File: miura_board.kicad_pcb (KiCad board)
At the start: 2 copper layers, 60 x 60 mm, 27 parts, among them J1 Conn_01x02_Female, J2 Screw_Terminal_01x02, J3 Screw_Terminal_01x02, SW1 SW_Push, U1 ATmega32U4-A, U2 NRF24L01, U3 DRV8833PW, U4 DRV8833PW, U5 ESP32-S2-SOLO, Y1 16MHz, Y2 16MHz

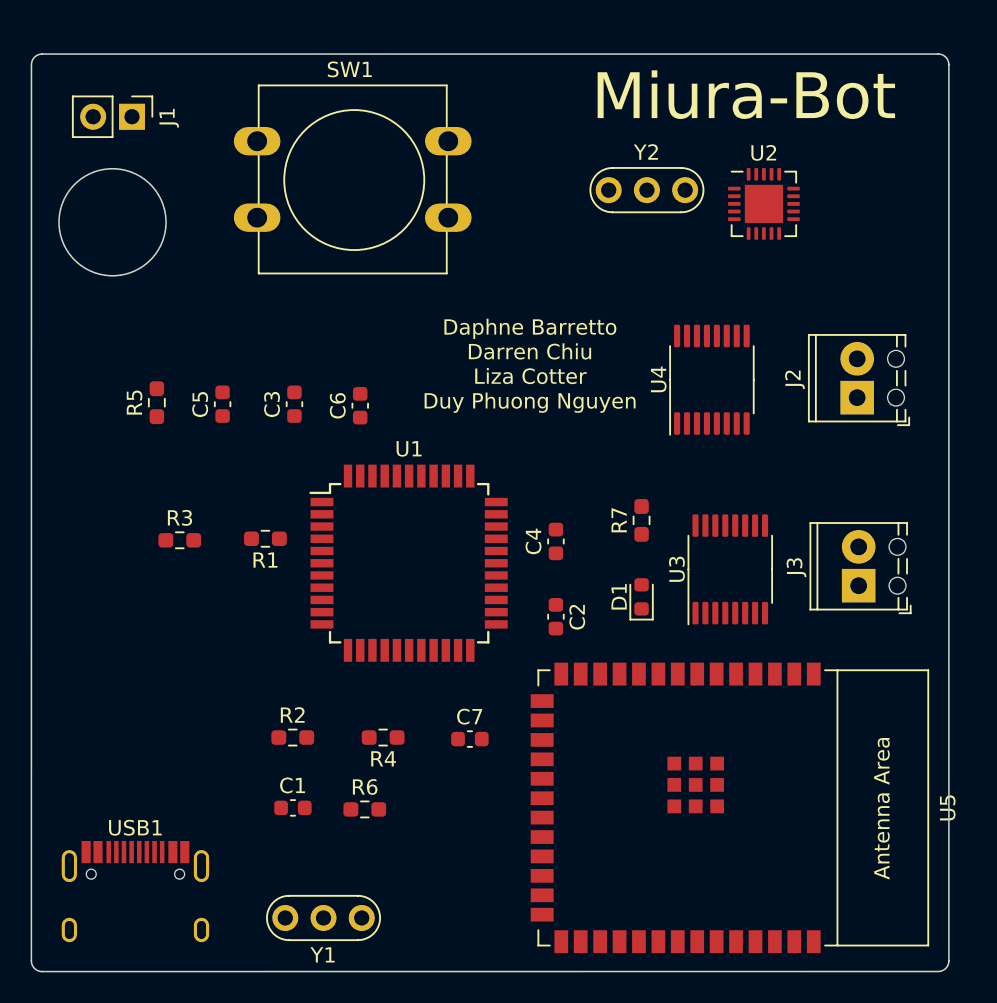
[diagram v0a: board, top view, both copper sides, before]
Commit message: STEP
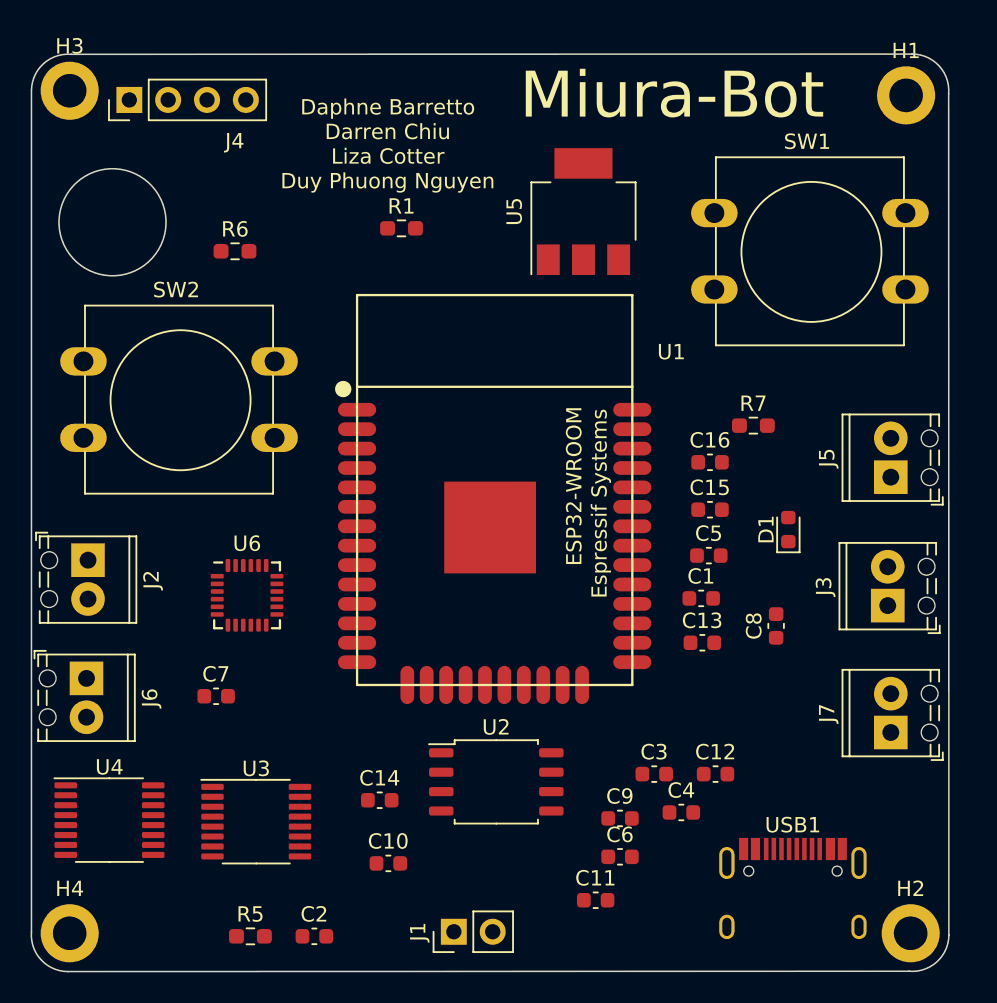
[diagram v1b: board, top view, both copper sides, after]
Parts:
- removed R2: 22, Resistor_SMD:R_0603_1608Metric_Pad0.98x0.95mm_HandSolder
- removed R3, R4: 10k, Resistor_SMD:R_0603_1608Metric_Pad0.98x0.95mm_HandSolder
- removed Y1, Y2: 16MHz, Crystal:Resonator-3Pin_W7.0mm_H2.5mm
- added C10: 0.1uF, Capacitor_SMD:C_0603_1608Metric, F.Cu at (84.3, 77.8)
- added C11: 0.1uF, Capacitor_SMD:C_0603_1608Metric, F.Cu at (97.9, 80.2)
- added C12: 0.1uF, Capacitor_SMD:C_0603_1608Metric, F.Cu at (105.7, 72.0)
- added C13: 0.1uF, Capacitor_SMD:C_0603_1608Metric, F.Cu at (104.9, 63.4)
- added C14: 0.1uF, Capacitor_SMD:C_0603_1608Metric, F.Cu at (83.8, 73.7)
- added C15: 0.1uF, Capacitor_SMD:C_0603_1608Metric, F.Cu at (105.4, 54.7)
- added C16: 0.1uF, Capacitor_SMD:C_0603_1608Metric, F.Cu at (105.4, 51.6)
- added C8: 10uF, Capacitor_SMD:C_0603_1608Metric, F.Cu at (109.7, 62.3)
- added C9: 10uF, Capacitor_SMD:C_0603_1608Metric, F.Cu at (99.5, 74.9)
- added H1: MountingHole_Pad, MountingHole:MountingHole_2.2mm_M2_DIN965_Pad, F.Cu at (118.2, 27.6)
- added H2: MountingHole_Pad, MountingHole:MountingHole_2.2mm_M2_DIN965_Pad, F.Cu at (118.5, 82.4)
- added H3: MountingHole_Pad, MountingHole:MountingHole_2.2mm_M2_DIN965_Pad, F.Cu at (63.5, 27.3)
- added H4: MountingHole_Pad, MountingHole:MountingHole_2.2mm_M2_DIN965_Pad, F.Cu at (63.5, 82.4)
- added J4: Conn_01x04_Male, Connector_PinHeader_2.54mm:PinHeader_1x04_P2.54mm_Vertical, F.Cu at (67.4, 27.9)
- added J5: Screw_Terminal_01x02, TerminalBlock_Phoenix:TerminalBlock_Phoenix_MPT-0,5-2-2.54_1x02_P2.54mm_Horizontal, F.Cu at (117.2, 52.6)
- added J6: Screw_Terminal_01x02, TerminalBlock_Phoenix:TerminalBlock_Phoenix_MPT-0,5-2-2.54_1x02_P2.54mm_Horizontal, F.Cu at (64.6, 65.7)
- added J7: Screw_Terminal_01x02, TerminalBlock_Phoenix:TerminalBlock_Phoenix_MPT-0,5-2-2.54_1x02_P2.54mm_Horizontal, F.Cu at (117.2, 69.3)
- added SW2: SW_Push, Button_Switch_THT:SW_PUSH-12mm, F.Cu at (64.4, 45.0)
- added U6: MPU-6050, Sensor_Motion:InvenSense_QFN-24_4x4mm_P0.5mm, F.Cu at (75.1, 60.3)
- C4: value 0.1uF -> 10uF
- R1: value 22 -> 10k
- U1: value ATmega32U4-A -> ESP32-WROOM; footprint Package_QFP:TQFP-44_10x10mm_P0.8mm -> ESP32-footprints-Lib:ESP32-WROOM
- U2: value NRF24L01 -> W25Q32JVSS; footprint Package_DFN_QFN:QFN-20-1EP_4x4mm_P0.5mm_EP2.5x2.5mm -> Package_SO:SOIC-8_5.23x5.23mm_P1.27mm
- U5: value ESP32-S2-SOLO -> AMS1117; footprint Espressif:ESP32-S2-SOLO -> Package_TO_SOT_SMD:SOT-223-3_TabPin2
- moved J1 57.3 mm to (88.6, 82.3), turned to 90 degrees
- moved J2 51.4 mm to (64.7, 58.0), turned to -90 degrees
- moved U4 48.8 mm to (66.1, 75.0), turned to 0 degrees
- moved USB1 43.0 mm to (110.8, 84.6)
- moved U2 41.7 mm to (91.4, 72.5)
- moved U5 39.6 mm to (97.1, 35.2), turned to 90 degrees
- moved R6 37.5 mm to (74.3, 37.8)
- moved R5 35.4 mm to (75.3, 82.6), turned to 0 degrees
- moved U3 35.1 mm to (75.7, 75.1), turned to 0 degrees
- moved C6 34.0 mm to (99.5, 77.4), turned to 0 degrees
- moved C3 33.7 mm to (101.7, 72.0), turned to 0 degrees
- moved C5 33.3 mm to (105.3, 57.7), turned to 0 degrees
- moved SW1 30.3 mm to (105.7, 35.3)
- moved C1 30.0 mm to (104.8, 60.5)
- moved C2 26.2 mm to (79.5, 82.6), turned to 0 degrees
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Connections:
- C1 pad 1: Net-(C1-Pad1) -> +5V
- C4 pad 1: XTAL1 -> +5V
- C7 pad 1: XTAL2 -> GND
- D1 pad 2: +5V -> +3V3
- J2 pad 1: unconnected-(J2-Pad1) -> Net-(U3-Pad7)
- J2 pad 2: unconnected-(J2-Pad2) -> Net-(U3-Pad5)
- J3 pad 1: unconnected-(J3-Pad1) -> Net-(U4-Pad2)
- J3 pad 2: unconnected-(J3-Pad2) -> Net-(U4-Pad4)
- R1 pad 1: D+ -> +3V3
- R1 pad 2: Net-(R1-Pad2) -> Net-(U1-Pad3)
- SW1 pad 1: GND -> Net-(U1-Pad3)
- SW1 pad 2: RESET -> GND
- U1 pad 1: unconnected-(U1-Pad1) -> GND
- U1 pad 10: unconnected-(U1-Pad10) -> MOTOR_B12_IN
- U1 pad 11: unconnected-(U1-Pad11) -> MOTOR_B11_IN
- U1 pad 12: unconnected-(U1-Pad12) -> MOTOR_A12_IN
- U1 pad 13: RESET -> MOTOR_A11_IN
- U1 pad 14: +5V -> unconnected-(U1-Pad14)
- U1 pad 16: XTAL2 -> unconnected-(U1-Pad16)
- U1 pad 17: XTAL1 -> unconnected-(U1-Pad17)
- U1 pad 19: unconnected-(U1-Pad19) -> SPI_CS
- U1 pad 2: +5V -> +3V3
- U1 pad 20: unconnected-(U1-Pad20) -> SPI_CLK
- U1 pad 21: unconnected-(U1-Pad21) -> MISO
- U1 pad 22: unconnected-(U1-Pad22) -> MOSI
- U1 pad 23: GND -> unconnected-(U1-Pad23)
- U1 pad 24: +5V -> unconnected-(U1-Pad24)
- U1 pad 25: unconnected-(U1-Pad25) -> Net-(U1-Pad25)
- U1 pad 3: Net-(R2-Pad1) -> Net-(U1-Pad3)
- U1 pad 33: Net-(R3-Pad1) -> SDA
- U1 pad 34: +5V -> RXD0
- U1 pad 35: GND -> TXD0
- U1 pad 36: unconnected-(U1-Pad36) -> SCL
- U1 pad 38: unconnected-(U1-Pad38) -> GND
- U1 pad 39: unconnected-(U1-Pad39) -> GND
- U1 pad 4: Net-(R1-Pad2) -> unconnected-(U1-Pad4)
- U1 pad 5: GND -> unconnected-(U1-Pad5)
- U1 pad 6: Net-(C1-Pad1) -> MOTOR_B22_IN
- U1 pad 7: unconnected-(U1-Pad7) -> MOTOR_B21_IN
- U1 pad 8: unconnected-(U1-Pad8) -> MOTOR_A22_IN
- U1 pad 9: unconnected-(U1-Pad9) -> MOTOR_A21_IN
- U2 pad 1: unconnected-(U2-Pad1) -> SPI_CS
- U2 pad 2: unconnected-(U2-Pad2) -> MISO
- U2 pad 4: unconnected-(U2-Pad4) -> GND
- U2 pad 5: unconnected-(U2-Pad5) -> MOSI
- U2 pad 6: unconnected-(U2-Pad6) -> SPI_CLK
- U2 pad 8: unconnected-(U2-Pad8) -> +3V3
- U3 pad 10: unconnected-(U3-Pad10) -> MOTOR_B12_IN
- U3 pad 12: unconnected-(U3-Pad12) -> MOTOR_SUPPLY
- U3 pad 15: unconnected-(U3-Pad15) -> MOTOR_A12_IN
- U3 pad 16: unconnected-(U3-Pad16) -> MOTOR_A11_IN
- U3 pad 2: unconnected-(U3-Pad2) -> Net-(U3-Pad2)
- U3 pad 4: unconnected-(U3-Pad4) -> Net-(U3-Pad4)
- U3 pad 5: unconnected-(U3-Pad5) -> Net-(U3-Pad5)
- U3 pad 7: unconnected-(U3-Pad7) -> Net-(U3-Pad7)
- U3 pad 9: unconnected-(U3-Pad9) -> MOTOR_B11_IN
- U4 pad 10: unconnected-(U4-Pad10) -> MOTOR_B22_IN
- U4 pad 12: unconnected-(U4-Pad12) -> MOTOR_SUPPLY
- U4 pad 15: unconnected-(U4-Pad15) -> MOTOR_A22_IN
- U4 pad 16: unconnected-(U4-Pad16) -> MOTOR_A21_IN
- U4 pad 2: unconnected-(U4-Pad2) -> Net-(U4-Pad2)
- U4 pad 4: unconnected-(U4-Pad4) -> Net-(U4-Pad4)
- U4 pad 5: unconnected-(U4-Pad5) -> Net-(U4-Pad5)
- U4 pad 7: unconnected-(U4-Pad7) -> Net-(U4-Pad7)
- U4 pad 9: unconnected-(U4-Pad9) -> MOTOR_B21_IN
- U5 pad 1: unconnected-(U5-Pad1) -> GND
- U5 pad 2: unconnected-(U5-Pad2) -> +3V3
- U5 pad 3: unconnected-(U5-Pad3) -> +5V
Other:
- outline, holes or cut-outs redrawn
